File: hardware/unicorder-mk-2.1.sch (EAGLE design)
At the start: 13 parts, among them IC1 TINY85

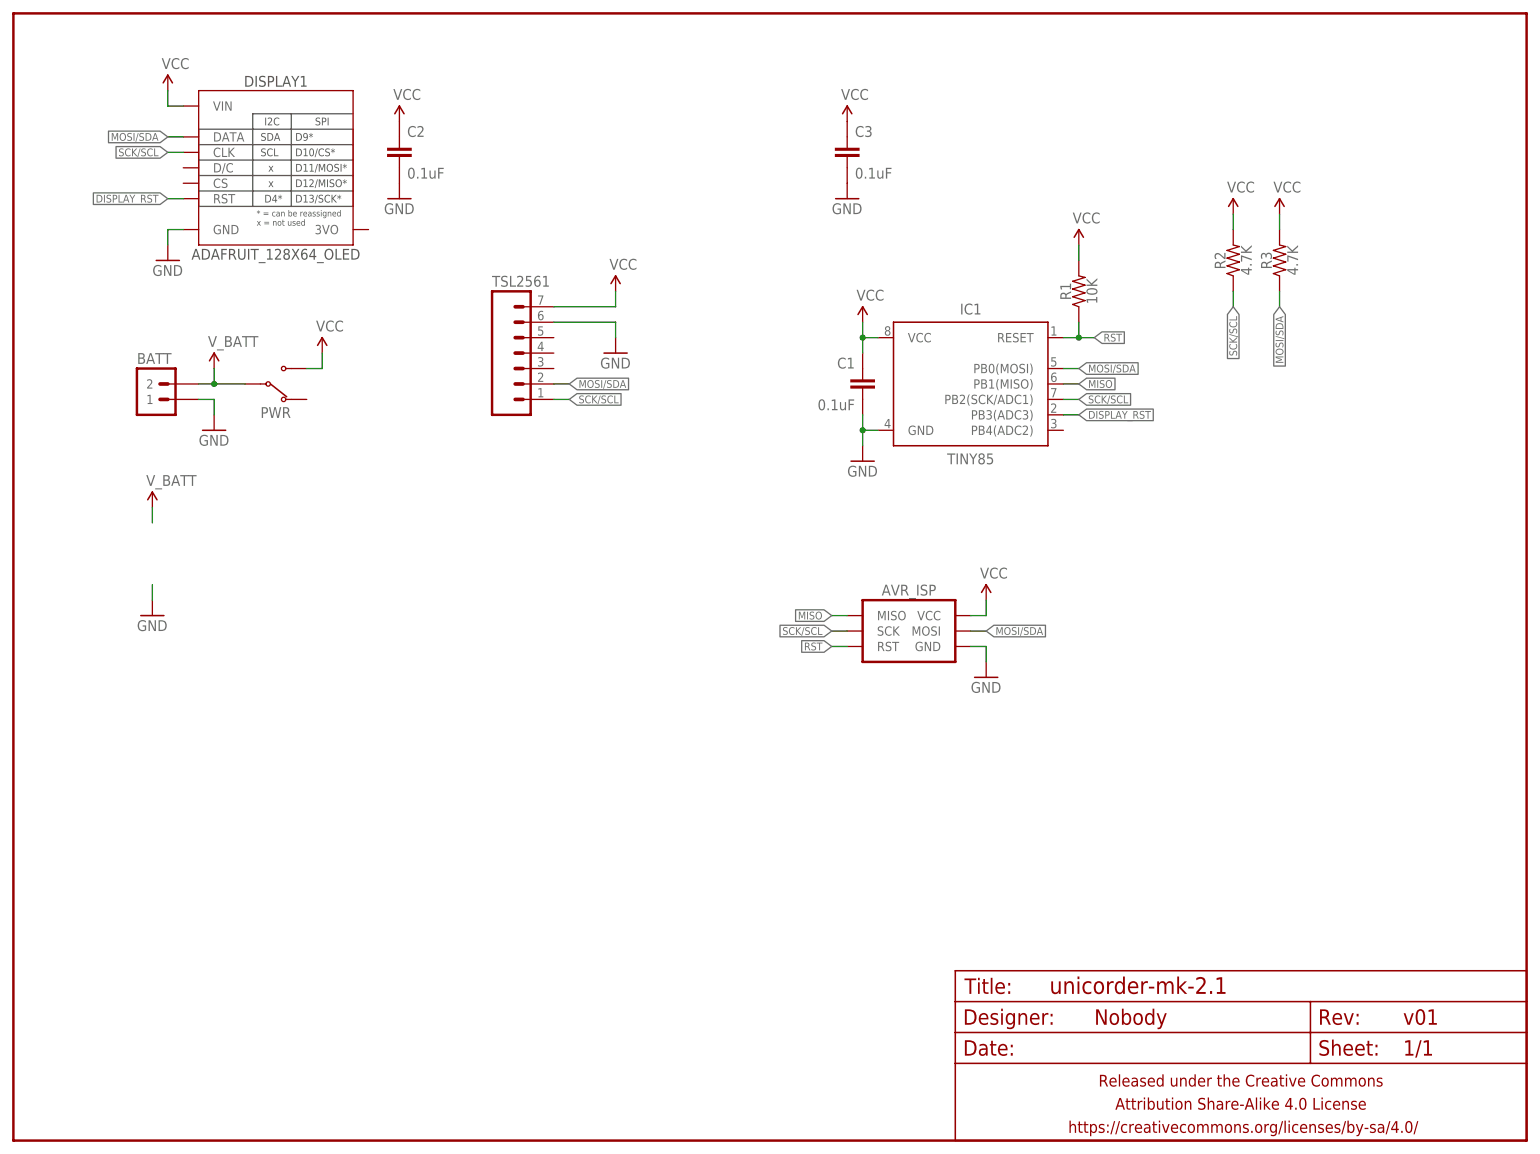
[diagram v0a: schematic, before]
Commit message: alsdkfjkalsdf
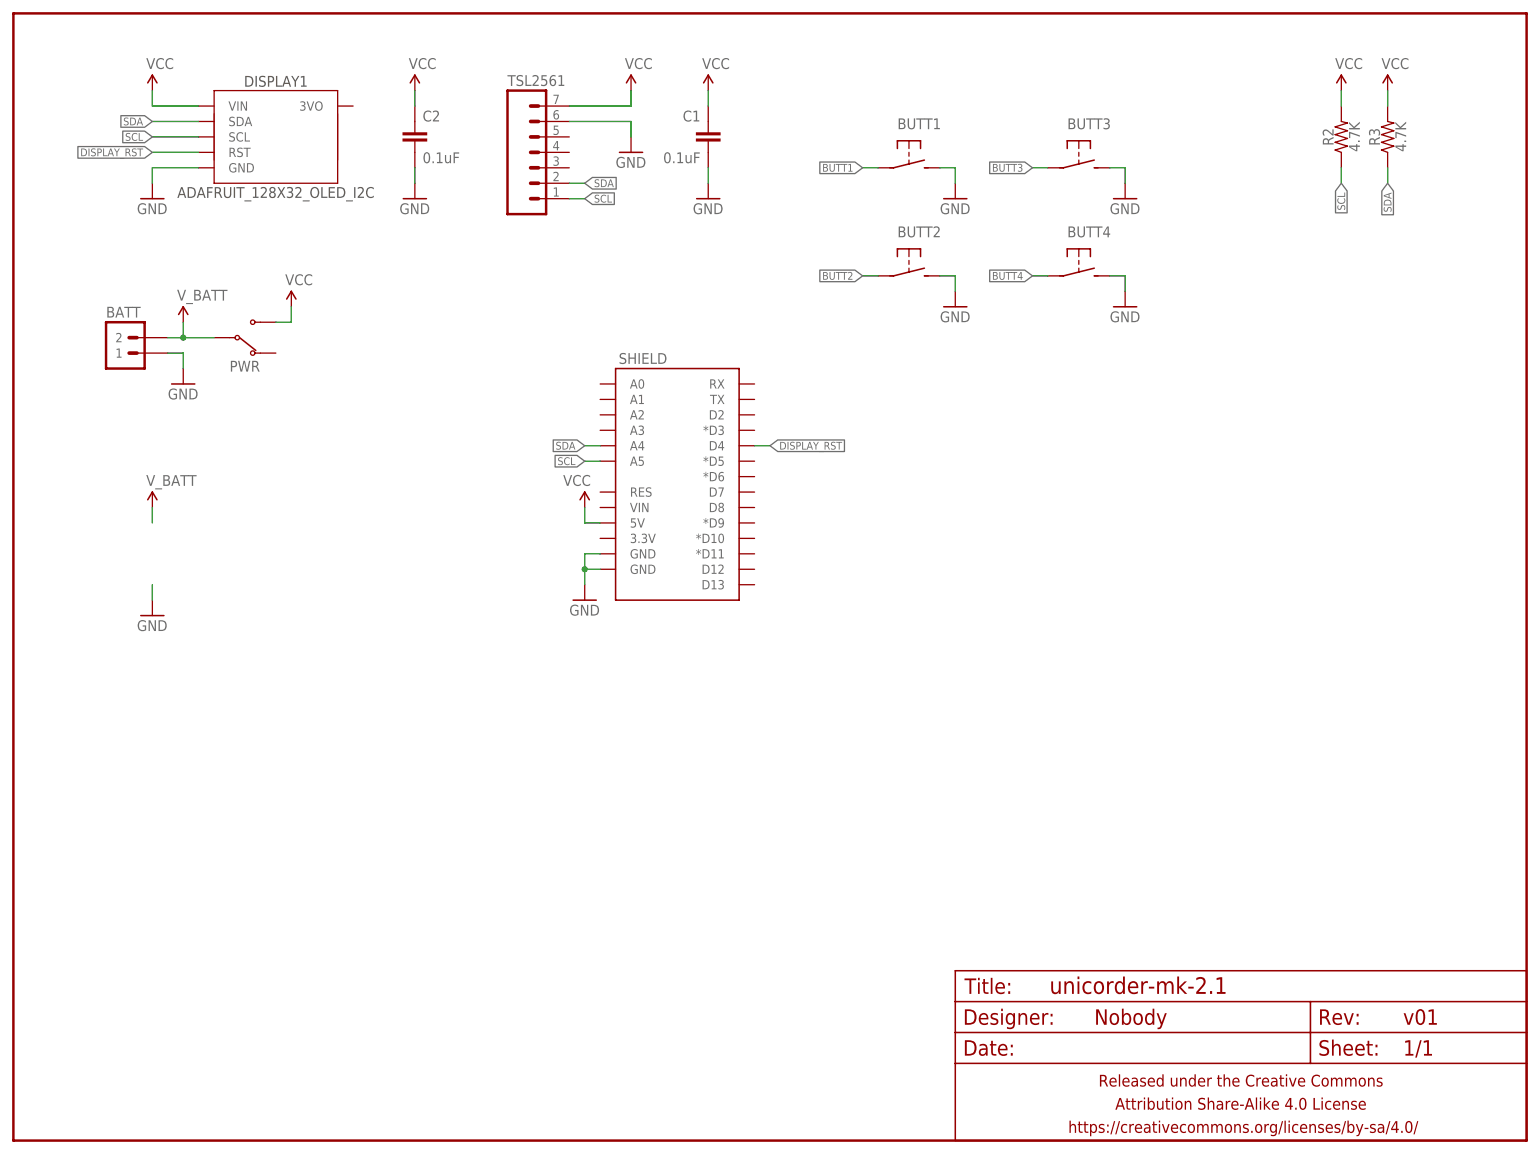
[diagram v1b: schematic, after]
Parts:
- removed AVR_ISP: AVR_SPI_PRG_6AVR-JST-PTH-RA-I2C, A_butts:AVR_SPI_PRG_6AVR-JST-PTH-RA-I2C
- removed C3: 0.1uF, A_butts:CAPACITOR-CERAMIC025-024X044
- removed IC1: TINY85, A_butts:ATTINY45TINY85-20-DIP
- removed R1: 10K, A_butts:RESISTORPTH-AXIAL-7.62MM
- added BUTT1, BUTT2, BUTT3, BUTT4: SPST-NO-TACT6MM-PTH-SMALL-PADS, A_butts:SPST-NO-TACT6MM-PTH-SMALL-PADS
- added SHIELD: (no value), A_butts:ARDUINO_SHIELD_SMALLER
- DISPLAY1: value ADAFRUIT_128X64_OLED -> ADAFRUIT_128X32_OLED_I2C; device A_butts:ADAFRUIT_128X64_OLED -> A_butts:ADAFRUIT_128X32_OLED_I2CCLOSER
- PWR: value SWITCH-SPDTPTH-RA-2MM -> SWITCH-SPDTPTH-VERT-2.54MM; device A_butts:SWITCH-SPDTPTH-RA-2MM -> A_butts:SWITCH-SPDTPTH-VERT-2.54MM
- R2, R3: device A_butts:RESISTORPTH-AXIAL-7.62MM -> A_butts:RESISTORPTH-AXIAL-6.35MM
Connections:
- removed net MISO: AVR_ISP.MISO, IC1.PB1(MISO)
- removed net MOSI/SDA: AVR_ISP.MOSI, DISPLAY1.DATA, IC1.PB0(MOSI), R3.1, TSL2561.2
- removed net RST: AVR_ISP.RST, IC1.RESET, R1.1
- removed net SCK/SCL: AVR_ISP.SCK, DISPLAY1.CLK, IC1.PB2(SCK/ADC1), R2.1, TSL2561.1
- new net BUTT1: BUTT1.1
- new net BUTT2: BUTT2.1
- new net BUTT3: BUTT3.1
- new net BUTT4: BUTT4.1
- new net SCL: DISPLAY1.SCL, R2.1, SHIELD.A5, TSL2561.1
- new net SDA: DISPLAY1.SDA, R3.1, SHIELD.A4, TSL2561.2
- net DISPLAY_RST: now also SHIELD.D4; no longer IC1.PB3(ADC3)
- net GND: now also BUTT1.2, BUTT2.2, BUTT3.2, BUTT4.2, SHIELD.GND@0, SHIELD.GND@1; no longer AVR_ISP.GND, C3.2, IC1.GND
- net VCC: now also SHIELD.5V; no longer AVR_ISP.VCC, C3.1, IC1.VCC, R1.2
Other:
- moved on the sheet: BATT, C1, C2, PWR, R2, R3, TSL2561
